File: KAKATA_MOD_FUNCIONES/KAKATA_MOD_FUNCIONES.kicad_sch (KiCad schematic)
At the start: 8 parts, among them U1 ESP32-S3-WROOM-1(N16R8)

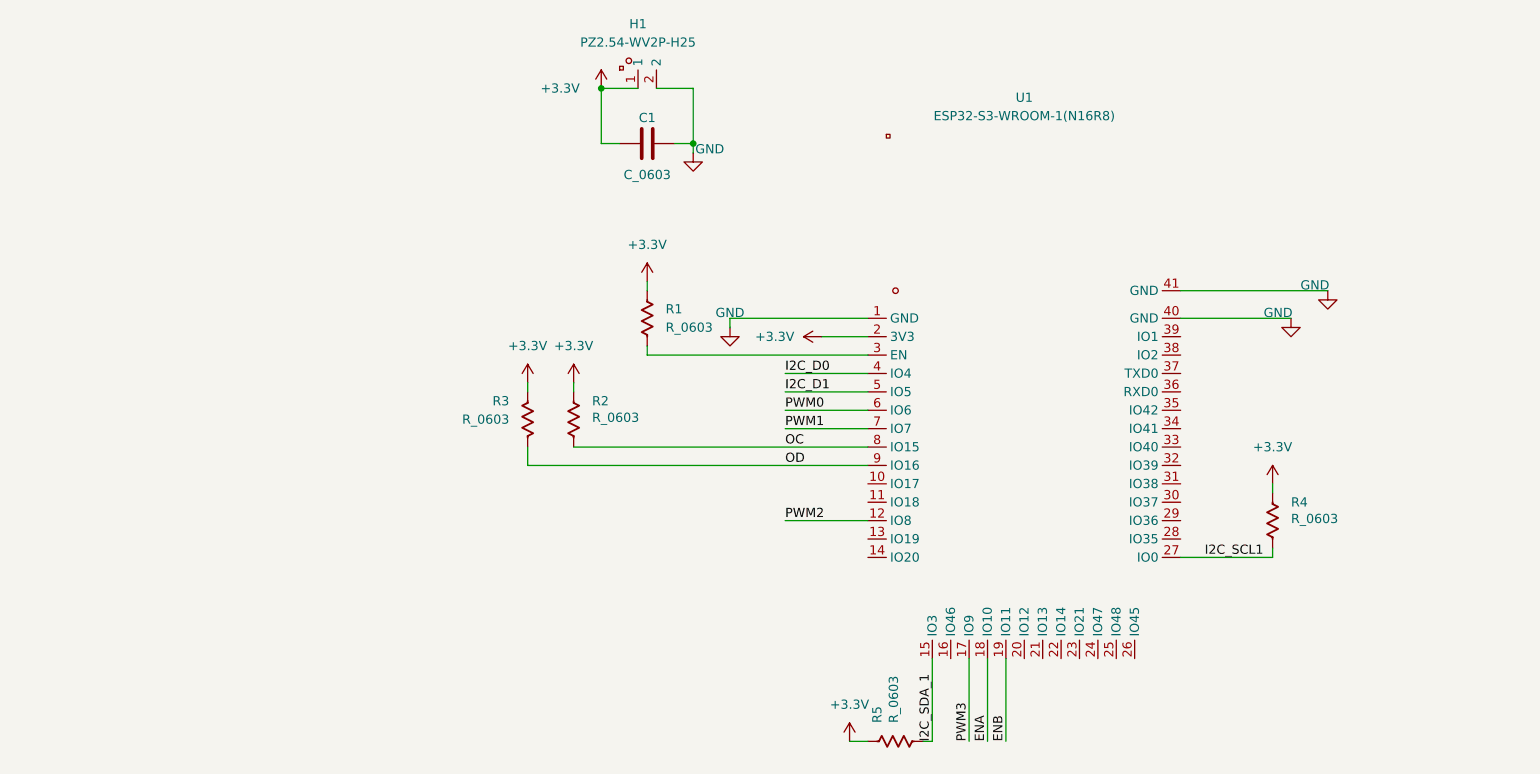
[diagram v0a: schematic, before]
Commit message: segundo commit
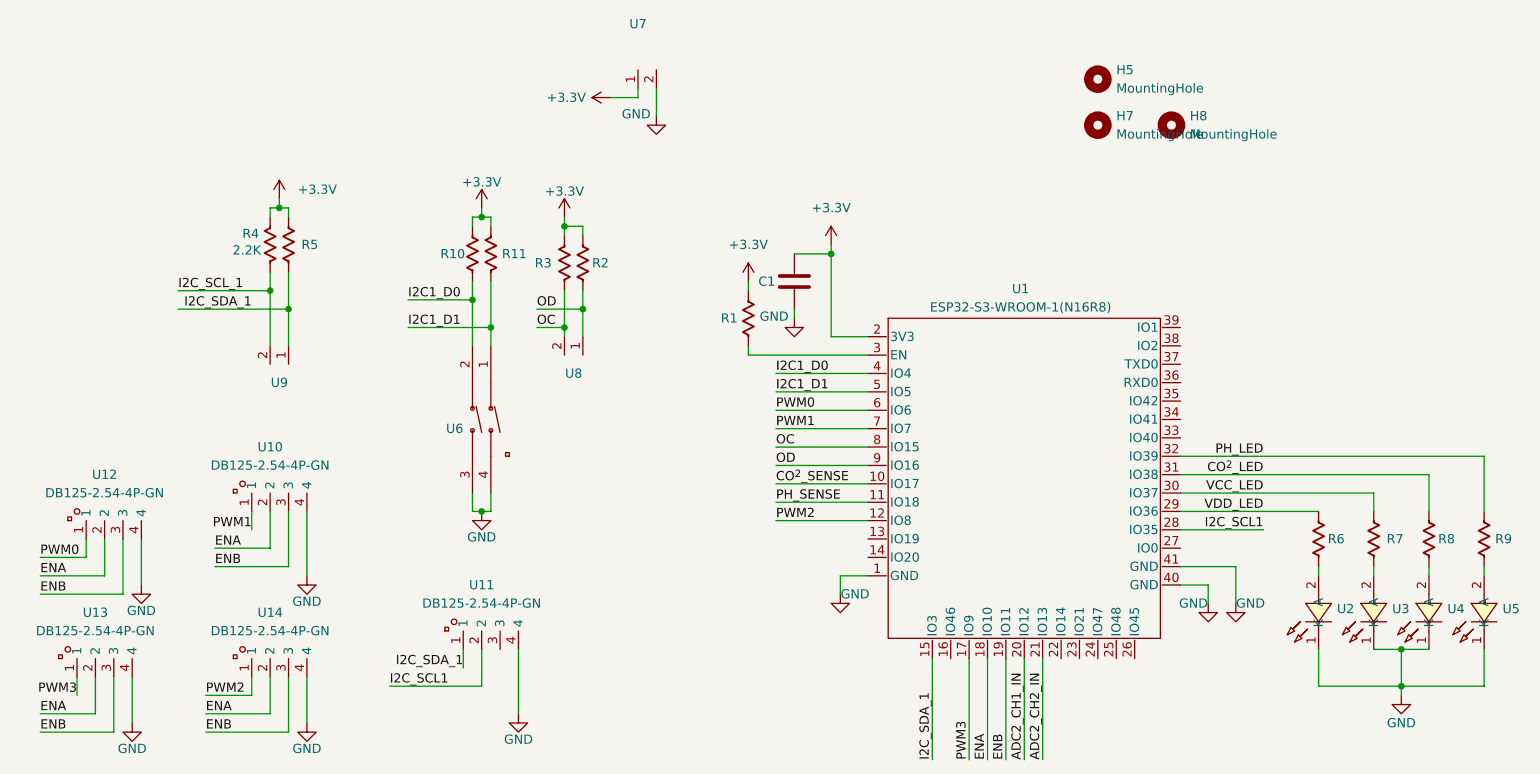
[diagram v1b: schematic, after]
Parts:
- removed H1: PZ2.54-WV2P-H25, EasyEDA:HDR-TH_2P-P2.54-V-M, symbol EasyEDA:PZ2.54-WV2P-H25
- added H5, H7, H8: MountingHole, MountingHole:MountingHole_2.2mm_M2, symbol Mechanical:MountingHole
- added R10, R11, R6, R7, R8, R9: R_0603, PCM_Resistor_SMD_AKL:R_0603_1608Metric, symbol PCM_Resistor_US_AKL:R_0603
- added U10, U11, U12, U13, U14: DB125-2.54-4P-GN, EasyEDA:CONN-TH_DB125-2.54-4P-GN, symbol EasyEDA:DB125-2.54-4P-GN
- added U2, U3, U4, U5: PSC-1608U52GC-G4, EasyEDA:LED0603-RD_GREEN, symbol EasyEDA:PSC-1608U52GC-G4
- added U6: SMQP-02R-TP, EasyEDA:SW-TH_4P-P2.54_SMQP-02R-TP, symbol EasyEDA:SMQP-02R-TP
- added U7, U8, U9: DB125-3.5-2P-GN-S, EasyEDA:CONN-TH_2P-P3.50_L7.4-W7.0, symbol EasyEDA:DB125-3.5-2P-GN-S
- R4, R5: value R_0603 -> 2.2K
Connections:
- net +3.3V: now also R10.2, R11.2, U7.1
- net ENA: now also U10.2, U12.2, U13.2, U14.2
- net ENB: now also U10.3, U12.3, U13.3, U14.3
- net GND: now also U10.4, U11.4, U12.4, U13.4, U14.4, U2.1 (K), U3.1 (K), U4.1 (K), U5.1 (K), U6.3, U6.4, U7.2
- net I2C_SCL1: now also U1.28 (IO35), U11.2; no longer R4.2, U1.27 (IO0)
- net I2C_SDA_1: now also U11.1, U9.1
- net OC: now also R3.2, U8.2; no longer R2.2
- net OD: now also R2.2, U8.1; no longer R3.2
- net PWM0: now also U12.1
- net PWM1: now also U10.1
- net PWM2: now also U14.1
- net PWM3: now also U13.1
- net CO^{2}_SENSE: now reaches U1.10 (IO17)
- net PH_SENSE: now reaches U1.11 (IO18)
- net ADC2_CH1_IN: now reaches U1.20 (IO12)
- net ADC2_CH2_IN: now reaches U1.21 (IO13)
- net VDD_LED: now reaches U1.29 (IO36)
- net VDD_LED: now also R6.1
- net VCC_LED: now reaches U1.30 (IO37)
- net VCC_LED: now also R7.1
- net CO^{2}_LED: now reaches U1.31 (IO38)
- net CO^{2}_LED: now also R8.1
- net PH_LED: now reaches U1.32 (IO39)
- net PH_LED: now also R9.1
- net I2C_D0 renamed I2C1_D0
- net I2C1_D0: now also R10.1, U6.2
- net I2C_D1 renamed I2C1_D1
- net I2C1_D1: now also R11.1, U6.1
- new net: R6.2, U2.2 (A)
- new net: R8.2, U4.2 (A)
- new net: R9.2, U5.2 (A)
- new net: R7.2, U3.2 (A)
- new net I2C_SCL_1: R4.2, U9.2
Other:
- moved on the sheet: C1, R1, R2, R3, R4, R5
